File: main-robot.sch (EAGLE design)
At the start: 71 parts, among them CON1 AX12, CON2 AX12, SW1 SWITCH-SPDT-H, SW2 PUSH-BUTTON436331045822, SW3 PUSH-BUTTON, SW4 PUSH-BUTTON, SW5 PUSH-BUTTON436331045822, SW6 PUSH-BUTTON436331045822, SW7 PUSH-BUTTON436331045822, U1 TEENSY_3.5_DIL+4

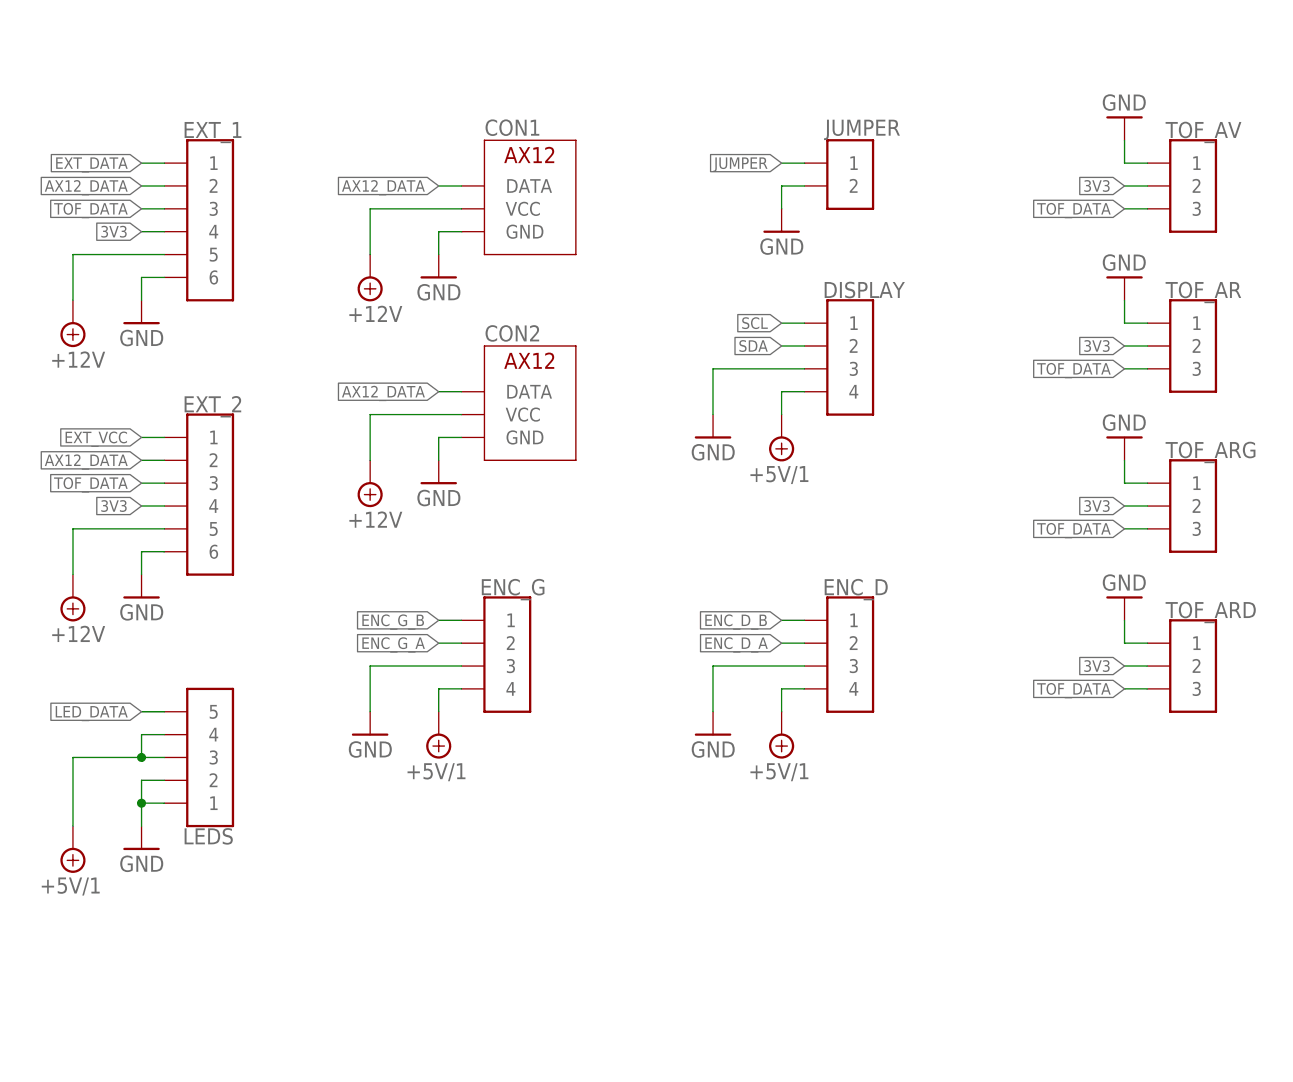
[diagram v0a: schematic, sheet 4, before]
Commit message: brd: begin routing
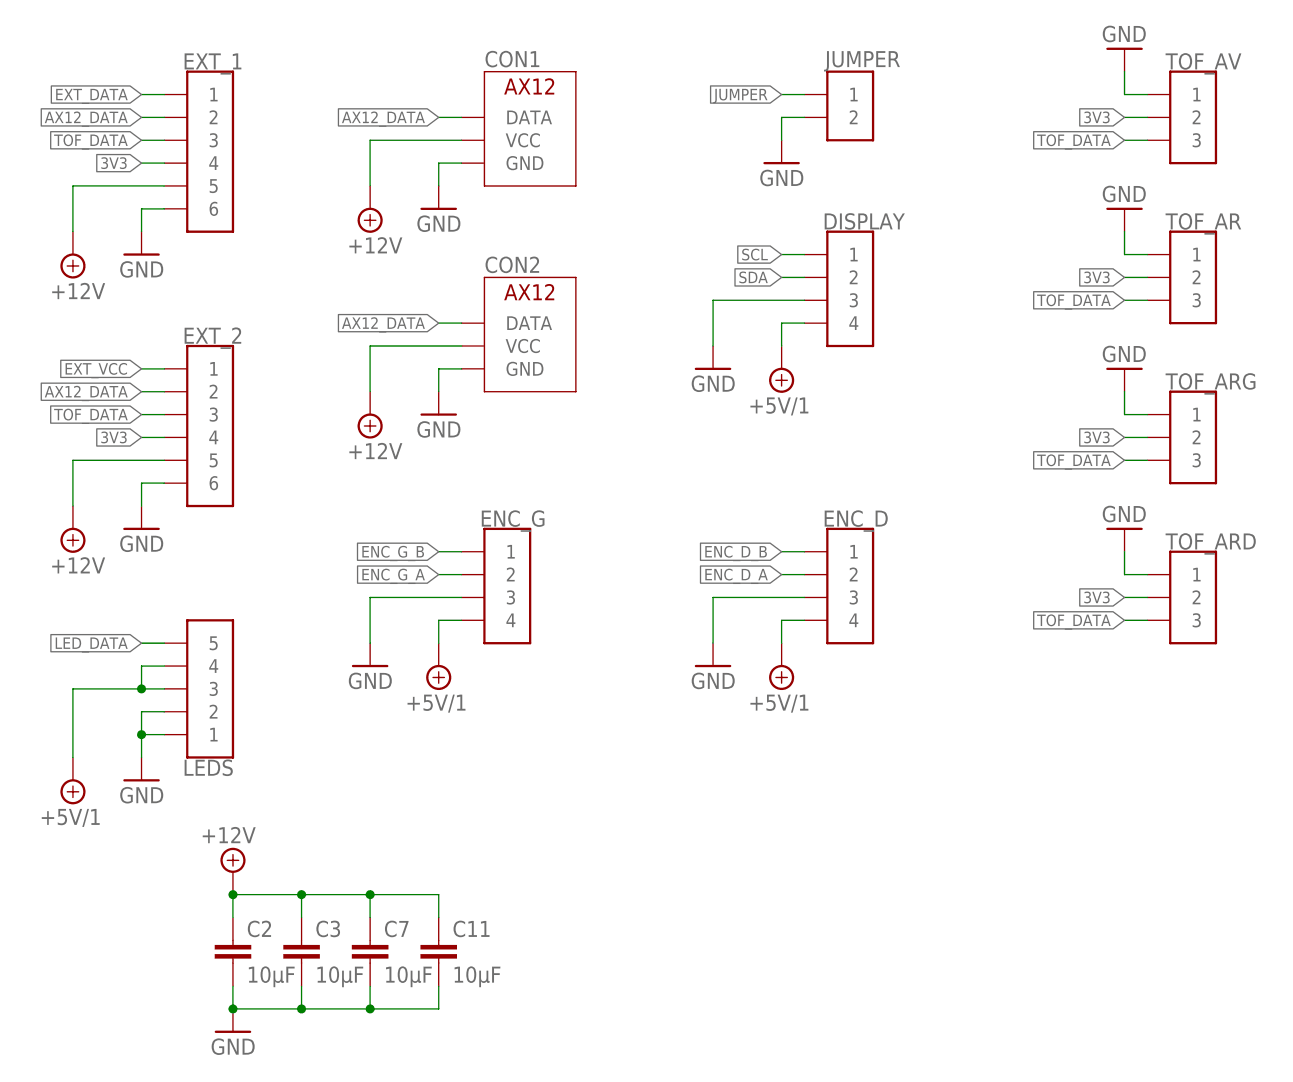
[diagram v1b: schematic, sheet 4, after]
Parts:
- added C11, C2, C3, C7: 10µF, resistor:C-EUC0805
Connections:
- net +12V: now also C11.1, C2.1, C3.1, C7.1
- net GND: now also C11.2, C2.2, C3.2, C7.1, C7.2
- net N$13: now also C7.2
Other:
- moved on the sheet: CON1, CON2, DISPLAY, ENC_D, ENC_G, EXT_1, EXT_2, JUMPER, LEDS, TOF_AR, TOF_ARD, TOF_ARG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

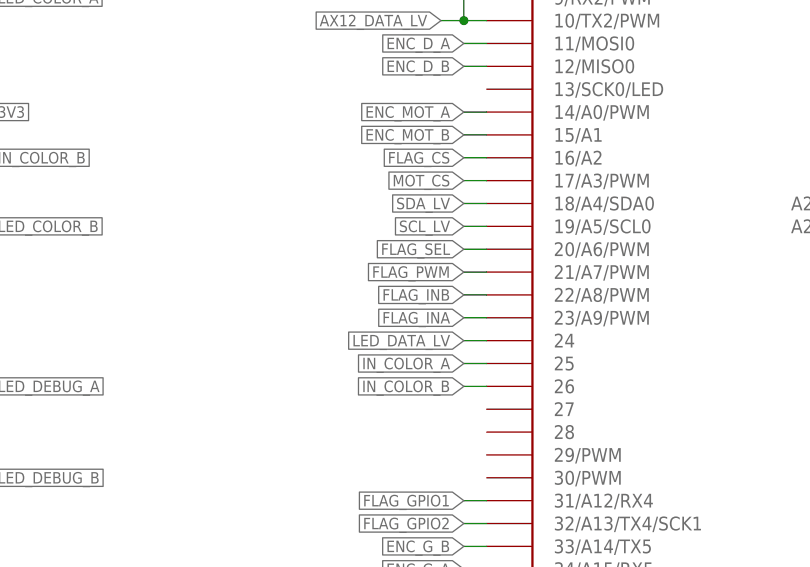
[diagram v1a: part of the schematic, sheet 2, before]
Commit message: routing in progress
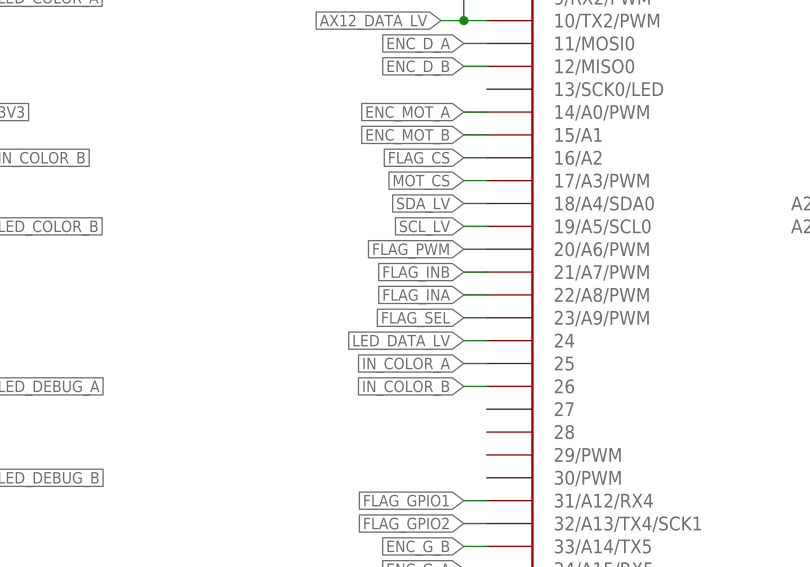
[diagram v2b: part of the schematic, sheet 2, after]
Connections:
- net FLAG_INA: now also U1.22/A8/PWM; no longer U1.23/A9/PWM
- net FLAG_INB: now also U1.21/A7/PWM; no longer U1.22/A8/PWM
- net FLAG_PWM: now also U1.20/A6/PWM; no longer U1.21/A7/PWM
- net FLAG_SEL: now also U1.23/A9/PWM; no longer U1.20/A6/PWM
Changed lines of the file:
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@@
 <net name="FLAG_INA" class="0">
-<segment>
-<pinref part="U1" gate="G$1" pin="23/A9/PWM"/>
-<wire x1="177.8" y1="91.44" x2="175.26" y2="91.44" width="0.1524" layer="91"/>
-<label x="175.26" y="91.44" size="1.27" layer="95" rot="R180" xref="yes"/>
-</segment>
-</net>
-<net name="FLAG_INB" class="0">
 <segment>
 <pinref part="U1" gate="G$1" pin="22/A8/PWM"/>
@@
 </segment>
 </net>
-<net name="FLAG_PWM" class="0">
+<net name="FLAG_INB" class="0">
 <segment>
 <pinref part="U1" gate="G$1" pin="21/A7/PWM"/>
@@
 </segment>
 </net>
-<net name="FLAG_SEL" class="0">
+<net name="FLAG_PWM" class="0">
 <segment>
 <pinref part="U1" gate="G$1" pin="20/A6/PWM"/>
@@
 </segment>
 </net>
+<net name="FLAG_SEL" class="0">
+<segment>
+<pinref part="U1" gate="G$1" pin="23/A9/PWM"/>
+<wire x1="177.8" y1="91.44" x2="175.26" y2="91.44" width="0.1524" layer="91"/>
+<label x="175.26" y="91.44" size="1.27" layer="95" rot="R180" xref="yes"/>
+</segment>
+</net>
